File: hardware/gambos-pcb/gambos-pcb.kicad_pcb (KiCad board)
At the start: 4 copper layers, 65 x 50 mm, 81 parts, among them J10 Conn_01x03_Pin, J11 Conn_01x03_Pin, J12 Conn_01x03_Pin, J13 Conn_01x03_Pin, J14 Conn_01x06_Pin, J15 Conn_01x01_Pin, J16 Conn_01x01_Pin, J17 Conn_01x01_Pin, J18 Conn_01x01_Pin, J19 Conn_01x01_Pin, J2 Conn_01x04_Pin, J20 Conn_01x01_Pin, J21 Conn_01x01_Pin, J22 Conn_01x01_Pin, J5 Conn_01x03_Pin, J7 Conn_01x03_Pin, J9 Conn_01x03_Pin, U1 STM32F446RET6U, U2 74AHCT244, U3 W25Q128JVS, U4 LSM6DS3, U5 BME280, U6 LIS3MDL, U8 MCP1825S, Y1 26MHz

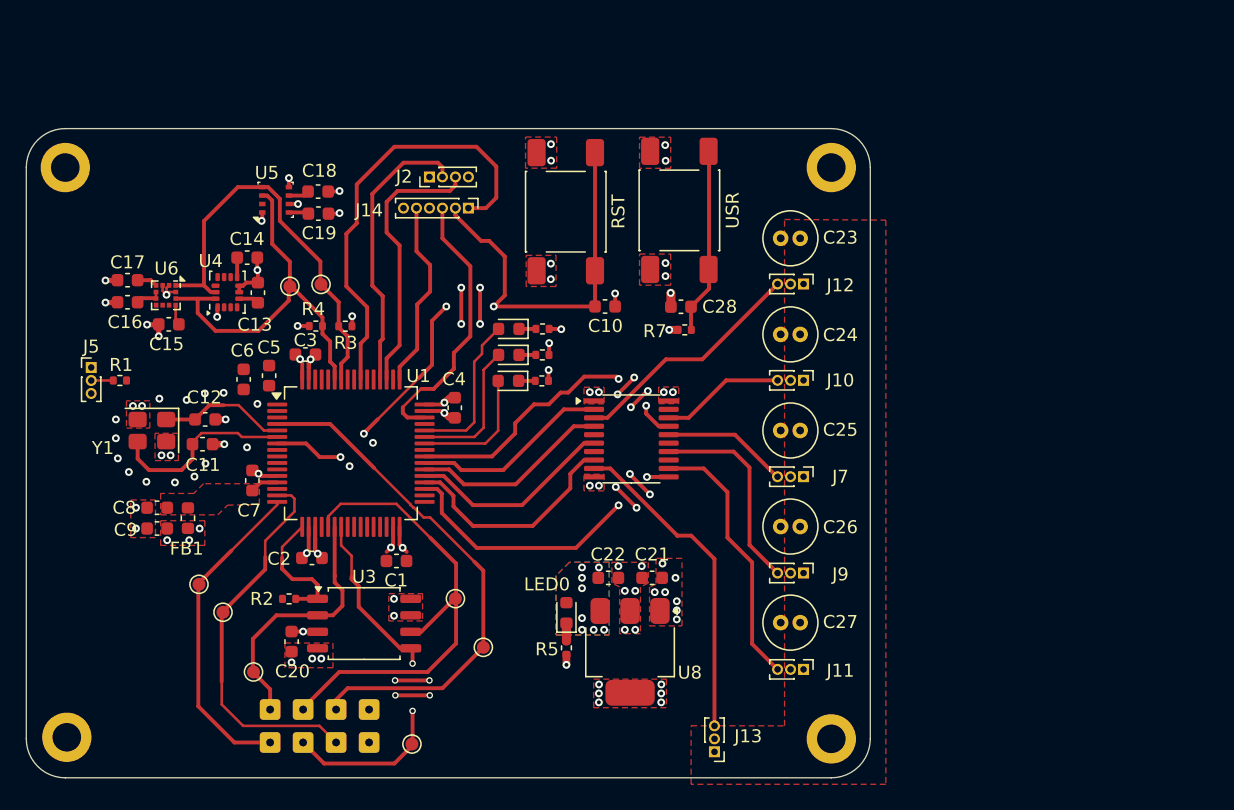
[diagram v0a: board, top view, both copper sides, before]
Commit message: Finished version before checks from hw engineers
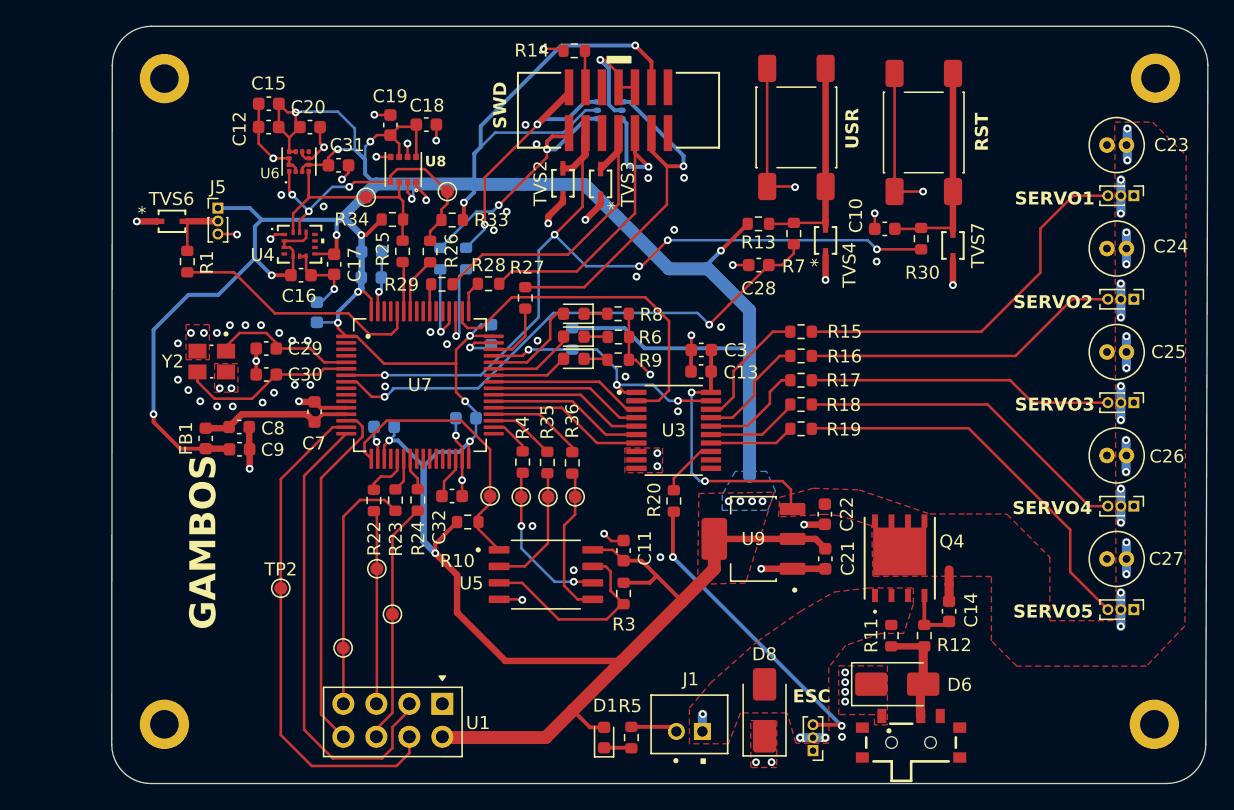
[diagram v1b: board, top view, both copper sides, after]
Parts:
- removed J14: Conn_01x06_Pin, Connector_PinHeader_1.00mm:PinHeader_1x06_P1.00mm_Vertical
- removed J15, J16, J17, J18, J19, J20, J21, J22: Conn_01x01_Pin, Connector_Wire:SolderWire-0.1sqmm_1x01_D0.4mm_OD1mm
- removed J2: Conn_01x04_Pin, Connector_PinHeader_1.00mm:PinHeader_1x04_P1.00mm_Vertical
- removed RST, USR: SW_Push, Button_Switch_SMD:SW_Push_1P1T_NO_E-Switch_TL3301NxxxxxG
- removed TP10, TP8: TestPoint, TestPoint:TestPoint_Pad_D1.0mm
- removed Y1: 26MHz, Crystal:Crystal_SMD_3225-4Pin_3.2x2.5mm
- added C29: 10p, Capacitor_SMD:C_0603_1608Metric, F.Cu at (93.1, 76.6)
- added C30: 10p, Capacitor_SMD:C_0603_1608Metric, F.Cu at (93.1, 78.6)
- added C31: 220n, Capacitor_SMD:C_0603_1608Metric, F.Cu at (98.6, 62.5)
- added C32: 4.7uF, Capacitor_SMD:C_0603_1608Metric, F.Cu at (107.4, 88.0)
- added C33: 100n, Capacitor_SMD:C_0603_1608Metric, B.Cu at (101.2, 69.2)
- added D6: SMAJ5.0CA, Diode_SMD:D_SMA, F.Cu at (141.7, 102.5)
- added D8: SMAJ5.0CA, Diode_SMD:D_SMA, F.Cu at (131.5, 104.5)
- added J1: JST-PH, gambos-pcb:JST-PH, F.Cu at (125.7, 105.6)
- added J3: 3220-14-0300-00, gambos-pcb:3220-14-0300-00, F.Cu at (120.2, 58.3)
- added Q4: DMP3010LPSQ-13, gambos-pcb:DMP3010LPSQ-13, F.Cu at (141.9, 92.8)
- added R10: 100k, Resistor_SMD:R_0603_1608Metric, F.Cu at (108.6, 90.0)
- added R11: 100k, Resistor_SMD:R_0603_1608Metric, F.Cu at (141.2, 98.7)
- added R12: 10k, Resistor_SMD:R_0603_1608Metric, F.Cu at (143.8, 98.7)
- added R13: 10k, Resistor_SMD:R_0603_1608Metric, F.Cu at (131.0, 67.0)
- added R14: 100R, Resistor_SMD:R_0603_1608Metric, F.Cu at (116.8, 53.7)
- added R15: 0R, Resistor_SMD:R_0603_1608Metric, F.Cu at (134.3, 75.3)
- added R16: 0R, Resistor_SMD:R_0603_1608Metric, F.Cu at (134.3, 77.2)
- added R17: 0R, Resistor_SMD:R_0603_1608Metric, F.Cu at (134.3, 79.1)
- added R18: 0R, Resistor_SMD:R_0603_1608Metric, F.Cu at (134.3, 81.0)
- added R19: 0R, Resistor_SMD:R_0603_1608Metric, F.Cu at (134.3, 82.8)
- added R20: 0R, Resistor_SMD:R_0603_1608Metric, F.Cu at (124.5, 88.4)
- added R22: 0R, Resistor_SMD:R_0603_1608Metric, F.Cu at (101.4, 88.3)
- added R23: 0R, Resistor_SMD:R_0603_1608Metric, F.Cu at (103.0, 88.3)
- added R24: 0R, Resistor_SMD:R_0603_1608Metric, F.Cu at (104.8, 88.3)
- added R25: 0R, Resistor_SMD:R_0603_1608Metric, F.Cu at (103.6, 69.2)
- added R26: 0R, Resistor_SMD:R_0603_1608Metric, F.Cu at (105.7, 69.2)
- added R27: 0R, Resistor_SMD:R_0603_1608Metric, F.Cu at (113.0, 72.7)
- added R28: 0R, Resistor_SMD:R_0603_1608Metric, F.Cu at (110.2, 71.7)
- added R29: 0R, Resistor_SMD:R_0603_1608Metric, F.Cu at (106.6, 71.7)
- added R30: 470R, Resistor_SMD:R_0603_1608Metric, F.Cu at (143.5, 68.2)
- added R31: 0R, Resistor_SMD:R_0603_1608Metric, B.Cu at (108.5, 69.7)
- added R32: 0R, Resistor_SMD:R_0603_1608Metric, B.Cu at (106.5, 69.7)
- added R33: 4k7, Resistor_SMD:R_0603_1608Metric, F.Cu at (107.4, 66.7)
- added R34: 4k7, Resistor_SMD:R_0603_1608Metric, F.Cu at (102.8, 66.7)
- added R35: 0R, Resistor_SMD:R_0603_1608Metric, F.Cu at (114.7, 85.4)
- added R36: 0R, Resistor_SMD:R_0603_1608Metric, F.Cu at (116.7, 85.4)
- added SW1: SW_Push, Button_Switch_SMD:SW_Push_1P1T_NO_E-Switch_TL3301NxxxxxG, F.Cu at (133.9, 59.6)
- added SW3: SW_Push, Button_Switch_SMD:SW_Push_1P1T_NO_E-Switch_TL3301NxxxxxG, F.Cu at (143.7, 60.0)
- added Slide_SW1: 450404015514, gambos-pcb:450404015514, F.Cu at (142.7, 107.0)
- added TP12: TestPoint, TestPoint:TestPoint_Pad_D1.0mm, F.Cu at (107.0, 64.5)
- added TP13: TestPoint, TestPoint:TestPoint_Pad_D1.0mm, F.Cu at (100.8, 65.0)
- added TP14: TestPoint, TestPoint:TestPoint_Pad_D1.0mm, F.Cu at (116.9, 88.1)
- added TP2: TestPoint, TestPoint:TestPoint_Pad_D1.0mm, F.Cu at (94.2, 95.1)
- added TVS2: DESD5V0U1BA-7, gambos-pcb:DESD5V0U1BA-7, F.Cu at (115.9, 63.9)
- added TVS3: DESD5V0U1BA-7, gambos-pcb:DESD5V0U1BA-7, F.Cu at (118.8, 64.0)
- added TVS4: DESD5V0U1BA-7, gambos-pcb:DESD5V0U1BA-7, F.Cu at (136.2, 68.3)
- added TVS6: DESD5V0U1BA-7, gambos-pcb:DESD5V0U1BA-7, F.Cu at (85.8, 66.8)
- added TVS7: DESD5V0U1BA-7, gambos-pcb:DESD5V0U1BA-7, F.Cu at (146.0, 68.7)
- added U7: STM32F446RET6, gambos-pcb:STM32F446RET6, F.Cu at (104.9, 79.5)
- added U9: LDL1117S33R, gambos-pcb:LDL1117S33R, F.Cu at (130.6, 91.3)
- added Y2: TSX-3225_26MHZ, gambos-pcb:XTAL_TSX-3225_26.0000MF09Z-AC0, F.Cu at (88.9, 77.6)
- C1, C2, C4, C5, C6: moved to B.Cu
- C11, C12: value 20p -> 100n
- C14: value 100n -> 0.1u
- C16: value 1u -> 100n
- C20: value 100n -> 10u
- C3: value 100n -> 1u
- R1, R7: footprint Resistor_SMD:R_0402_1005Metric -> Resistor_SMD:R_0603_1608Metric
- R2: value 100k -> 10K; footprint Resistor_SMD:R_0402_1005Metric -> Resistor_SMD:R_0603_1608Metric; moved to B.Cu
- R3: value 4k2 -> 10k; footprint Resistor_SMD:R_0402_1005Metric -> Resistor_SMD:R_0603_1608Metric
- R4: value 4k2 -> 0R; footprint Resistor_SMD:R_0402_1005Metric -> Resistor_SMD:R_0603_1608Metric
- R5: value 1k5 -> 260R; footprint Resistor_SMD:R_0402_1005Metric -> Resistor_SMD:R_0603_1608Metric
- R6, R8, R9: value 130R -> 260R; footprint Resistor_SMD:R_0402_1005Metric -> Resistor_SMD:R_0603_1608Metric
- U1: value STM32F446RET6U -> NRF24L01_Breakout; footprint Package_QFP:LQFP-64_10x10mm_P0.5mm -> RF_Module:nRF24L01_Breakout
- U2: value 74AHCT244 -> D1213A-04S-7; footprint Package_SO:SSOP-20_4.4x6.5mm_P0.65mm -> gambos-pcb:D1213A-04S-7; moved to B.Cu
- U3: value W25Q128JVS -> SN74HCT541PWR; footprint Package_SO:SOIC-8_5.3x5.3mm_P1.27mm -> gambos-pcb:SOP65P640X120-20N
- U4: value LSM6DS3 -> LSM6DSVTR; footprint Package_LGA:LGA-14_3x2.5mm_P0.5mm_LayoutBorder3x4y -> gambos-pcb:LSM6DSVTR
- U5: value BME280 -> W25Q128JVSIQ; footprint Package_LGA:Bosch_LGA-8_2.5x2.5mm_P0.65mm_ClockwisePinNumbering -> gambos-pcb:W25Q128JVSIQ
- U6: value LIS3MDL -> LIS2MDLTR; footprint Package_LGA:LGA-12_2x2mm_P0.5mm -> gambos-pcb:LIS2MDLTR
- U8: value MCP1825S -> BME280; footprint Package_TO_SOT_SMD:SOT-223-3_TabPin2 -> gambos-pcb:BME280
- moved H4 83.8 mm to (161.5, 105.6)
- moved C14 60.5 mm to (145.7, 96.9), turned to 90 degrees
- moved H3 51.4 mm to (85.2, 105.6)
- moved U8 41.0 mm to (103.6, 62.9)
- moved C20 39.7 mm to (96.5, 59.6), turned to 0 degrees
- moved J12 35.7 mm to (159.9, 96.7)
- moved U5 35.6 mm to (114.6, 94.0), turned to 0 degrees
- moved C13 34.7 mm to (126.6, 78.4), turned to 180 degrees
- moved C11 33.8 mm to (120.6, 92.2), turned to 90 degrees
- moved C3 30.5 mm to (126.6, 76.8), turned to 180 degrees
- moved R3 29.7 mm to (120.6, 95.5), turned to -90 degrees
- moved R2 29.6 mm to (116.7, 75.9), turned to -90 degrees
- moved J10 29.1 mm to (159.9, 64.9)
- moved J7 28.9 mm to (159.9, 72.8)
- moved J9 28.6 mm to (159.9, 80.8)
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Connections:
- net /MCU/PWR_LED_MINUS renamed Net-(D1-K)
- net /Sensors and flash/INT1_ACC renamed /Schematic/Sensors and flash/INT1
- net /Sensors and flash/INT2_GYRO renamed /Schematic/Sensors and flash/INT2
- net /Sensors and flash/INT_MAG renamed /Schematic/Sensors and flash/INT/DRDY
- C10 pad 1: NRST -> TVS_NRST
- C11 pad 1: /MCU/HSE_IN -> +3V3
- C12 pad 1: /MCU/HSE_OUT -> +3V3
- C13 pad 1: +3V3 -> +5V
- C14 pad 1: +3V3 -> Net-(Q4-G)
- C14 pad 2: GND -> +5V
- C17 pad 1: Net-(U6-C1) -> +3V3
- C21 pad 1: /MCU/V_IN -> +3V3
- C22 pad 1: +3V3 -> +5V
- C28 pad 1: USER_BTN -> /Schematic/Microcontroller/USER_BTN
- C3 pad 1: +3V3 -> +5V
- D2 pad 2: USER_LED1 -> /Schematic/Microcontroller/USER_LED1
- D3 pad 2: USER_LED2 -> /Schematic/Microcontroller/USER_LED2
- D4 pad 2: USER_LED3 -> /Schematic/Microcontroller/USER_LED3
- J10 pad 3: PWM3_1_5V -> /Schematic/Servos and connectors/SERVO1_OUT
- J11 pad 3: PWM12_1_5V -> /Schematic/Servos and connectors/SERVO4_OUT
- J12 pad 3: PWM12_2_5V -> /Schematic/Servos and connectors/SERVO5_OUT
- J13 pad 2: +5V -> /Schematic/Power and ESC/V_IN
- J13 pad 3: PWM3_4_5V -> /Schematic/Servos and connectors/ESC_OUT
- J5 pad 2: /MCU/BOOT0 -> TVS_BOOT0
- J7 pad 3: PWM3_2_5V -> /Schematic/Servos and connectors/SERVO2_OUT
- J9 pad 3: PWM3_3_5V -> /Schematic/Servos and connectors/SERVO3_OUT
- R1 pad 1: /MCU/BOOT0 -> TVS_BOOT0
- R1 pad 2: /MCU/BOOT0 -> /Schematic/Microcontroller/BOOT0
- R2 pad 2: FLASH_CS -> ~BUFF_EN
- R3 pad 2: SCL -> Net-(U5-HOLD/RESET(IO3))
- R4 pad 1: +3V3 -> Net-(U7-PB13)
- R4 pad 2: SDA -> /Schematic/SPI2.SCK_2
- R7 pad 1: USER_BTN -> TVS_USER_BTN
- R7 pad 2: GND -> /Schematic/Microcontroller/USER_BTN
- TP3 pad 1: SCK_1 -> /Schematic/SPI1.SCK_1
- TP4 pad 1: SDA -> /Schematic/SPI1.MISO_1
- TP5 pad 1: MOSI_1 -> /Schematic/SPI1.MOSI_1
- TP6 pad 1: MISO_1 -> /Schematic/SPI2.SCK_2
- TP7 pad 1: SCL -> /Schematic/SPI2.MISO_2
- TP9 pad 1: NRF24_CE_SLD -> FLASH_CS
- U1 pad 1: +3V3 -> GND
- U1 pad 2: unconnected-(U1-PC13-Pad2) -> +3V3
- U1 pad 3: unconnected-(U1-PC14-Pad3) -> NRF24_CE_SLD
- U1 pad 4: NRF24_CE_SLD -> NRF24_CS_SLD
- U1 pad 5: /MCU/HSE_IN -> /Schematic/SPI1.SCK_1
- U1 pad 6: /MCU/HSE_OUT -> /Schematic/SPI1.MOSI_1
- U1 pad 7: NRST -> /Schematic/SPI1.MISO_1
- U1 pad 8: unconnected-(U1-PC0-Pad8) -> IRQ_SLD
- U2 pad 1: GND -> SWDIO
- U2 pad 2: PWM3_3_3V3 -> GND
- U2 pad 3: PWM12_2_5V -> SWCLK
- U2 pad 4: PWM3_2_3V3 -> UART4_RX
- U2 pad 5: unconnected-(U2-2Y1-Pad5) -> +3V3
- U2 pad 6: PWM3_1_3V3 -> UART4_TX
- U3 pad 1: FLASH_CS -> ~BUFF_EN
- U3 pad 2: MISO_1 -> /Schematic/Microcontroller/PWMs.SERVO1_IN
- U3 pad 3: +3V3 -> /Schematic/Microcontroller/PWMs.SERVO2_IN
- U3 pad 4: GND -> /Schematic/Microcontroller/PWMs.SERVO3_IN
- U3 pad 5: MOSI_1 -> /Schematic/Microcontroller/PWMs.SERVO4_IN
- U3 pad 6: SCK_1 -> /Schematic/Microcontroller/PWMs.SERVO5_IN
- U3 pad 7: +3V3 -> /Schematic/Microcontroller/PWMs.ESC_IN
- U3 pad 8: +3V3 -> GND
- U4 pad 13: SCL -> /Schematic/I2C.SCL
- U4 pad 14: SDA -> /Schematic/I2C.SDA
- U5 pad 1: GND -> FLASH_CS
- U5 pad 2: +3V3 -> /Schematic/SPI2.MISO_2
- U5 pad 3: SDA -> Net-(U5-HOLD/RESET(IO3))
- U5 pad 4: SCL -> GND
- U5 pad 5: GND -> /Schematic/SPI2.MOSI_2
- U5 pad 6: +3V3 -> /Schematic/SPI2.SCK_2
- U5 pad 7: GND -> Net-(U5-HOLD/RESET(IO3))
- U6 pad 1: SCL -> /Schematic/I2C.SCL
- U6 pad 11: SDA -> GND
- U6 pad 3: GND -> +3V3
- U6 pad 4: Net-(U6-C1) -> /Schematic/I2C.SDA
- U6 pad 6: +3V3 -> GND
- U6 pad 8: /Sensors and flash/DRDY_MAG -> GND
- U6 pad 9: GND -> +3V3
- U8 pad 1: /MCU/V_IN -> GND
- U8 pad 2: GND -> +3V3
- U8 pad 3: +3V3 -> /Schematic/I2C.SDA
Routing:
- net +3V3: track 23.8 -> 325.2 mm, vias 20 -> 22
- net GND: track 54.8 -> 122.8 mm, vias 91 -> 87
- net +5V: track 0.00 -> 48.3 mm, vias 2 -> 22
- net /Schematic/Microcontroller/USER_BTN: track 0.00 -> 41.2 mm, vias 0 -> 2
- net SCK_1: track 37.8 -> 0.00 mm
- net SDA: track 32.5 -> 0.00 mm
- net SCL: track 31.8 -> 0.00 mm
- net /Schematic/Servos and connectors/SERVO5_OUT: track 0.00 -> 30.5 mm
- net MOSI_1: track 29.3 -> 0.00 mm, vias 2 -> 0
- net /Schematic/Servos and connectors/SERVO1_OUT: track 0.00 -> 29.1 mm
- net /Schematic/Microcontroller/PWMs.SERVO1_IN: track 0.00 -> 26.9 mm
- net /Schematic/Servos and connectors/SERVO4_OUT: track 0.00 -> 26.0 mm
- net PWM3_4_5V: track 25.0 -> 0.00 mm
- net /Schematic/Servos and connectors/SERVO2_OUT: track 0.00 -> 24.6 mm
- net /Schematic/Servos and connectors/ESC_OUT: track 0.00 -> 24.2 mm, vias 0 -> 2
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- added copper zone on F.Cu, net /Schematic/Power and ESC/V_IN
- removed copper zone on F.Cu, net +3.3VA
- removed copper zone on F.Cu, net /MCU/V_IN
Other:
- board size 65 x 50 mm -> 84.4 x 58.3 mm
- board text added: "ESC"
- board text added: "GAMBOS"
- board text added: "RST"
- board text added: "SERVO1"
- board text added: "SERVO2"
- board text added: "SERVO3"
- board text added: "SERVO4"
- board text added: "SERVO5"
- board text added: "SWD"
- board text added: "USR"
